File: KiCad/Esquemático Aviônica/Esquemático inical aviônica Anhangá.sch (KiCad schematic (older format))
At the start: 20 parts, among them J1 Conn_01x06_Female, J2 Conn_01x06_Female, J3 Conn_01x12_Female, J4 Conn_01x12_Female, J5 Screw_Terminal_01x02, J6 Conn_01x06_Male, J7 Screw_Terminal_01x02, J8 Conn_01x07_Female, Q1 IRF7403, U1 ME620933

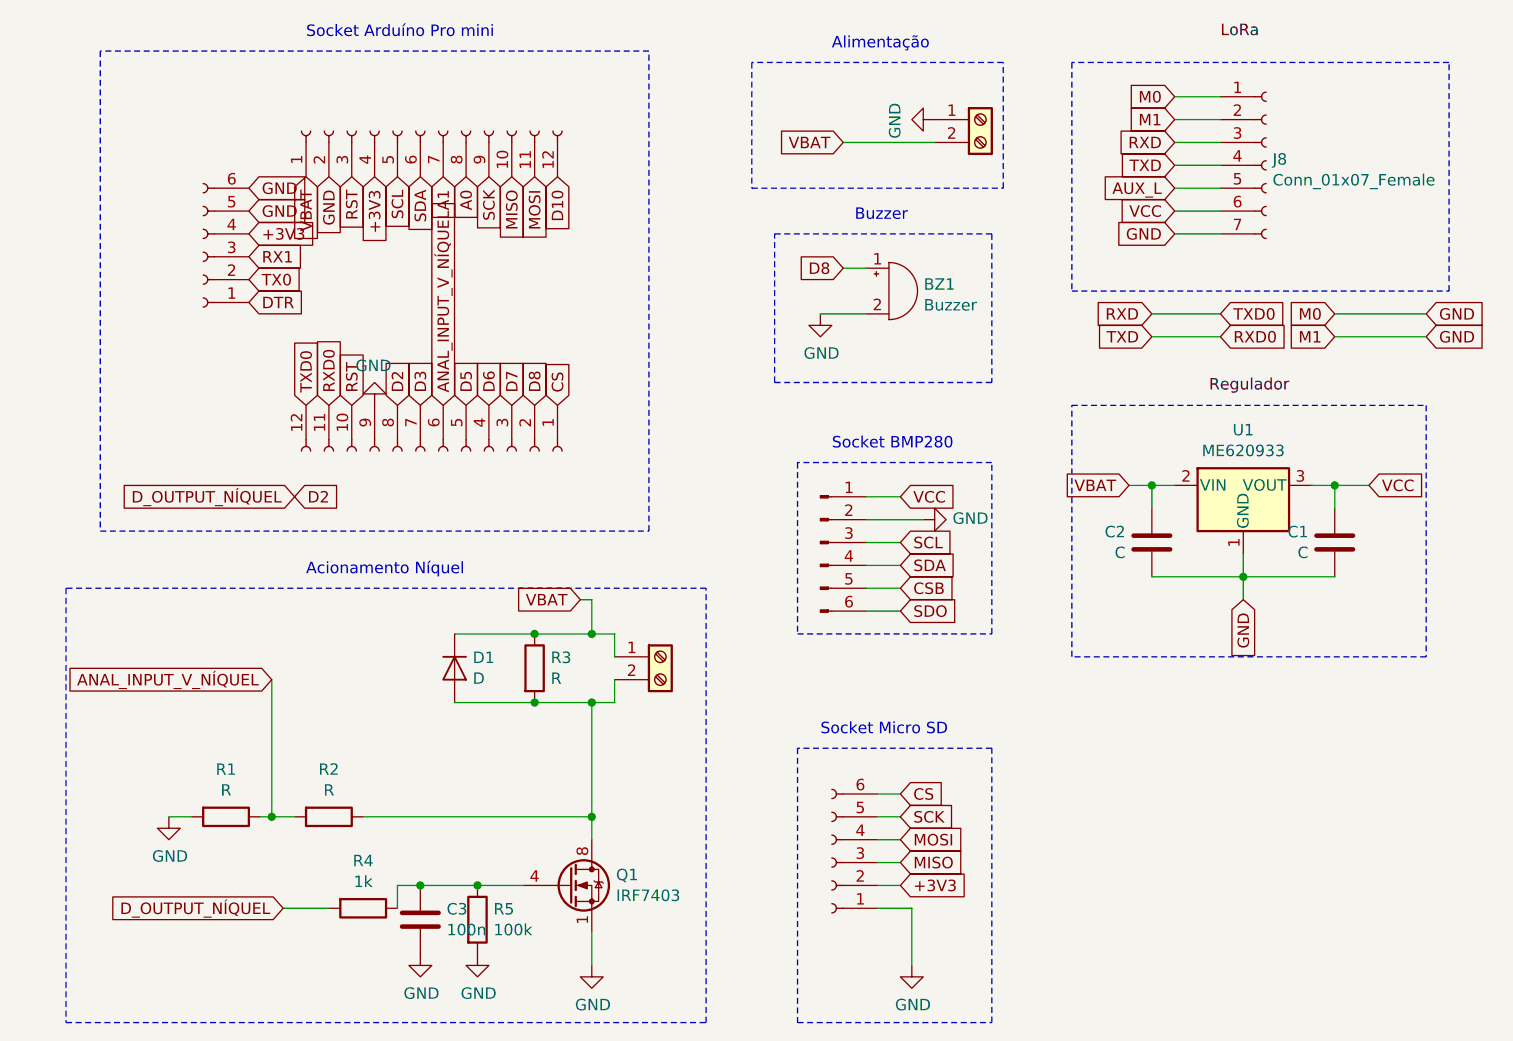
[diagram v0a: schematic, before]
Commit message: Revisão pós montagem
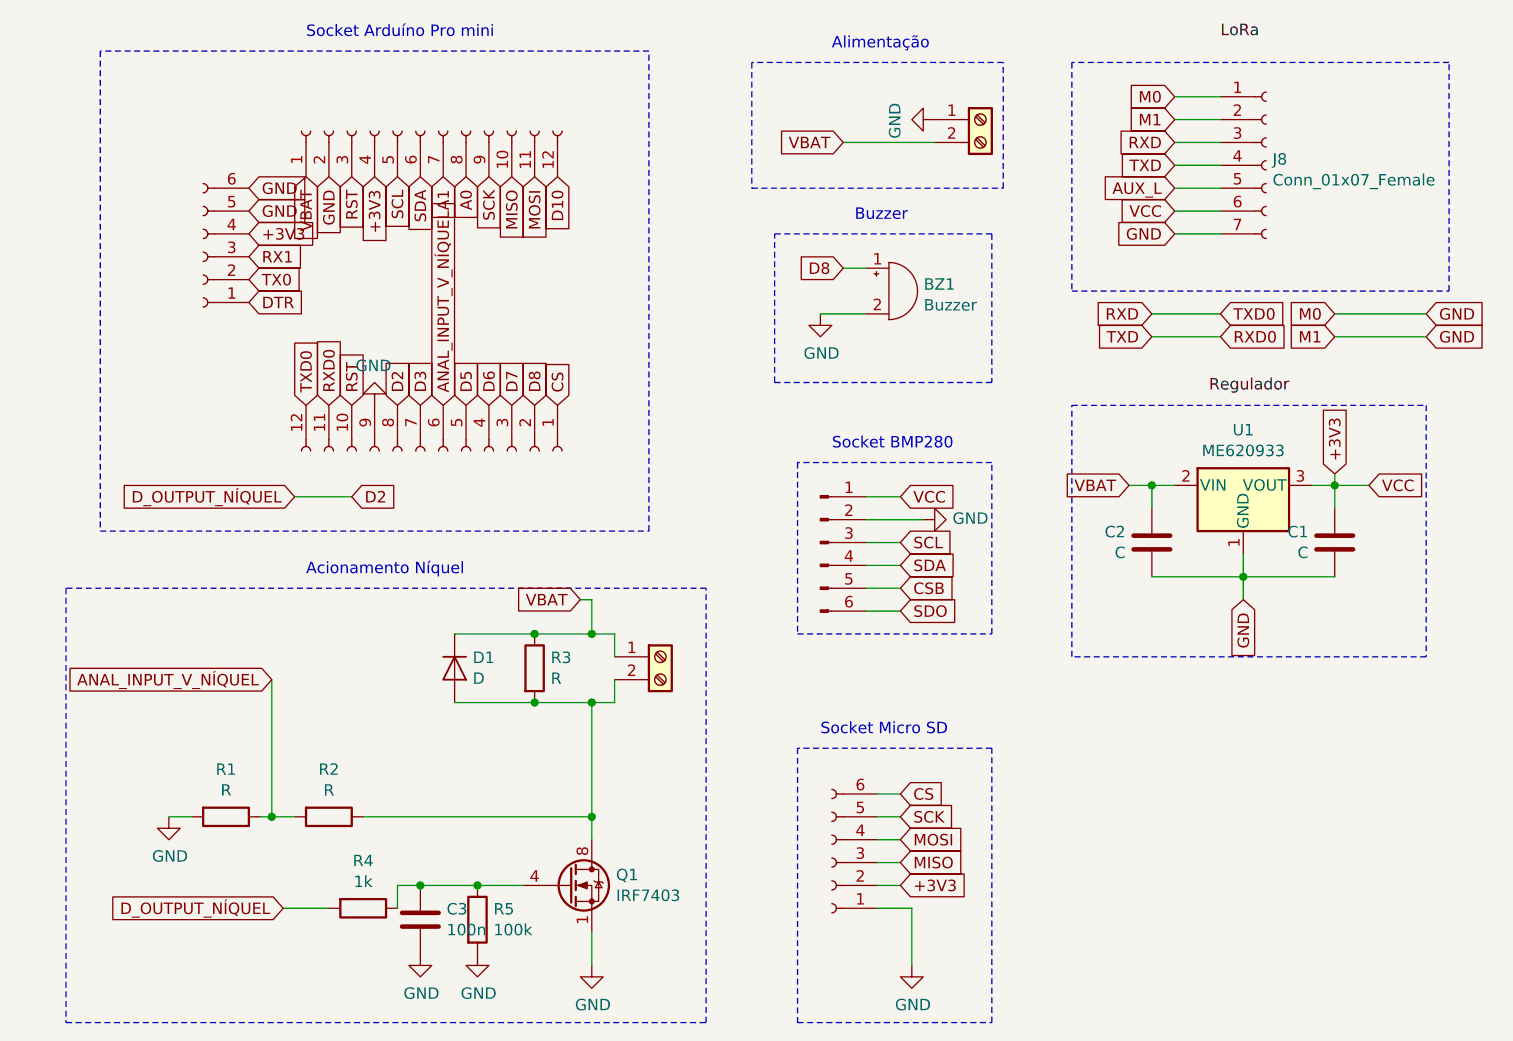
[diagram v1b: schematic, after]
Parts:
- J5, J7: footprint TerminalBlock_4Ucon:TerminalBlock_4Ucon_1x02_P3.50mm_Horizontal -> TerminalBlock:TerminalBlock_bornier-2_P5.08mm
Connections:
- net VCC is gone; now on net +3V3: C1.1, J6.1 (Pin_1), J8.6 (Pin_6), U1.3 (VOUT)
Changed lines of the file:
@@
 F 0 "J5" H 3980 5042 50  0001 L CNN
 F 1 "Screw_Terminal_01x02" H 3980 4951 50  0001 L CNN
-F 2 "TerminalBlock_4Ucon:TerminalBlock_4Ucon_1x02_P3.50mm_Horizontal" H 3900 5050 50  0001 C CNN
+F 2 "TerminalBlock:TerminalBlock_bornier-2_P5.08mm" H 3900 5050 50  0001 C CNN
 F 3 "~" H 3900 5050 50  0001 C CNN
 	1    3900 5050
@@
 F 0 "J7" H 5380 2692 50  0001 L CNN
 F 1 "Screw_Terminal_01x02" H 5380 2601 50  0001 L CNN
-F 2 "TerminalBlock_4Ucon:TerminalBlock_4Ucon_1x02_P3.50mm_Horizontal" H 5300 2700 50  0001 C CNN
+F 2 "TerminalBlock:TerminalBlock_bornier-2_P5.08mm" H 5300 2700 50  0001 C CNN
 F 3 "~" H 5300 2700 50  0001 C CNN
 	1    5300 2700
@@
 Text GLabel 2300 4350 0    50   Input ~ 0
 D_OUTPUT_NÍQUEL
-Text GLabel 2300 4350 2    50   Input ~ 0
+Text GLabel 2550 4350 2    50   Input ~ 0
 D2
 Text GLabel 3350 3950 1    50   Input ~ 0
@@
 Text GLabel 4700 3350 0    50   Input ~ 0
 D8
+Wire Wire Line
+	2300 4350 2550 4350
+Text GLabel 6850 4250 1    50   Input ~ 0
++3V3
+Wire Wire Line
+	6850 4250 6850 4300
 $EndSCHEMATC
